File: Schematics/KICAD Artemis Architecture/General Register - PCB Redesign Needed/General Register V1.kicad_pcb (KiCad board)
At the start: 4 copper layers, 54.8 x 34.2 mm, 24 parts, among them J1 Power, J2 Bus, J3 Control, J4 A Value, U4 74LS173, U5 74LS173, U6 74LS245

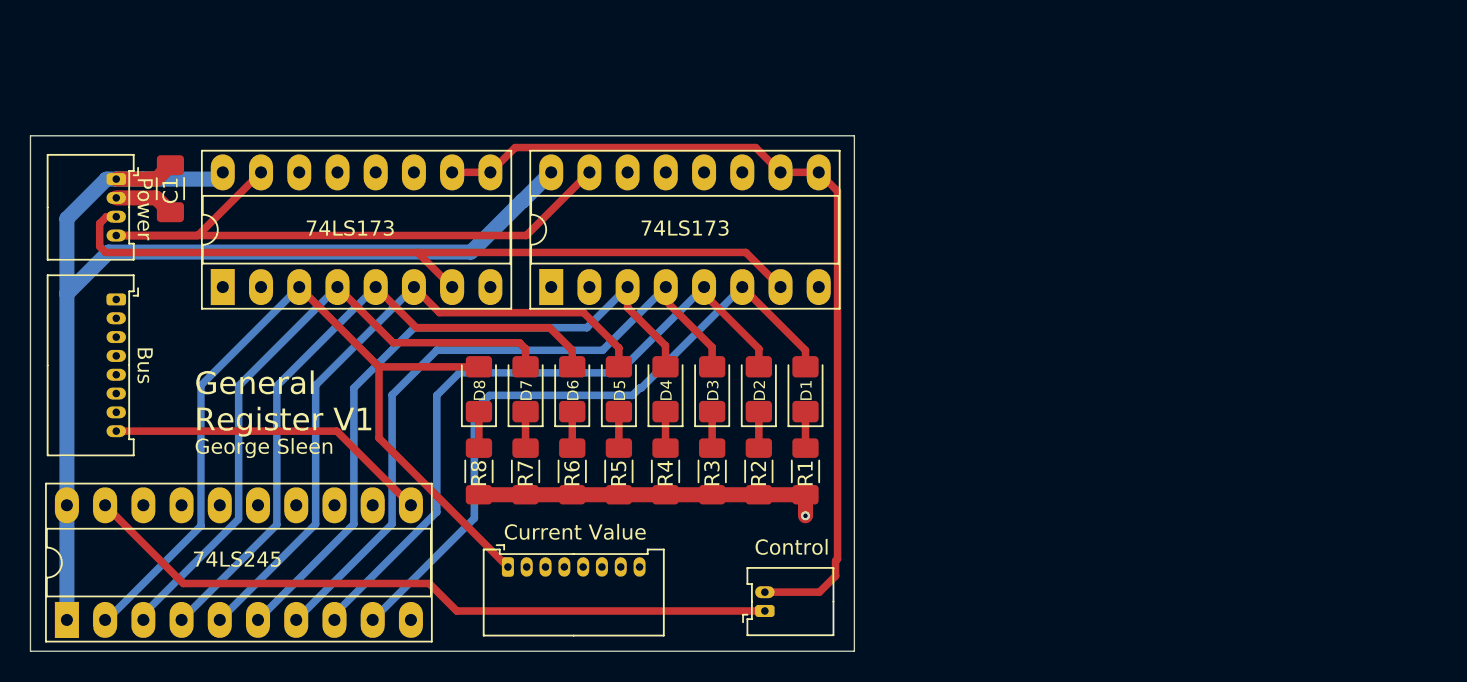
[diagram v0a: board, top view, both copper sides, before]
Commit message: Remade General Register PCB
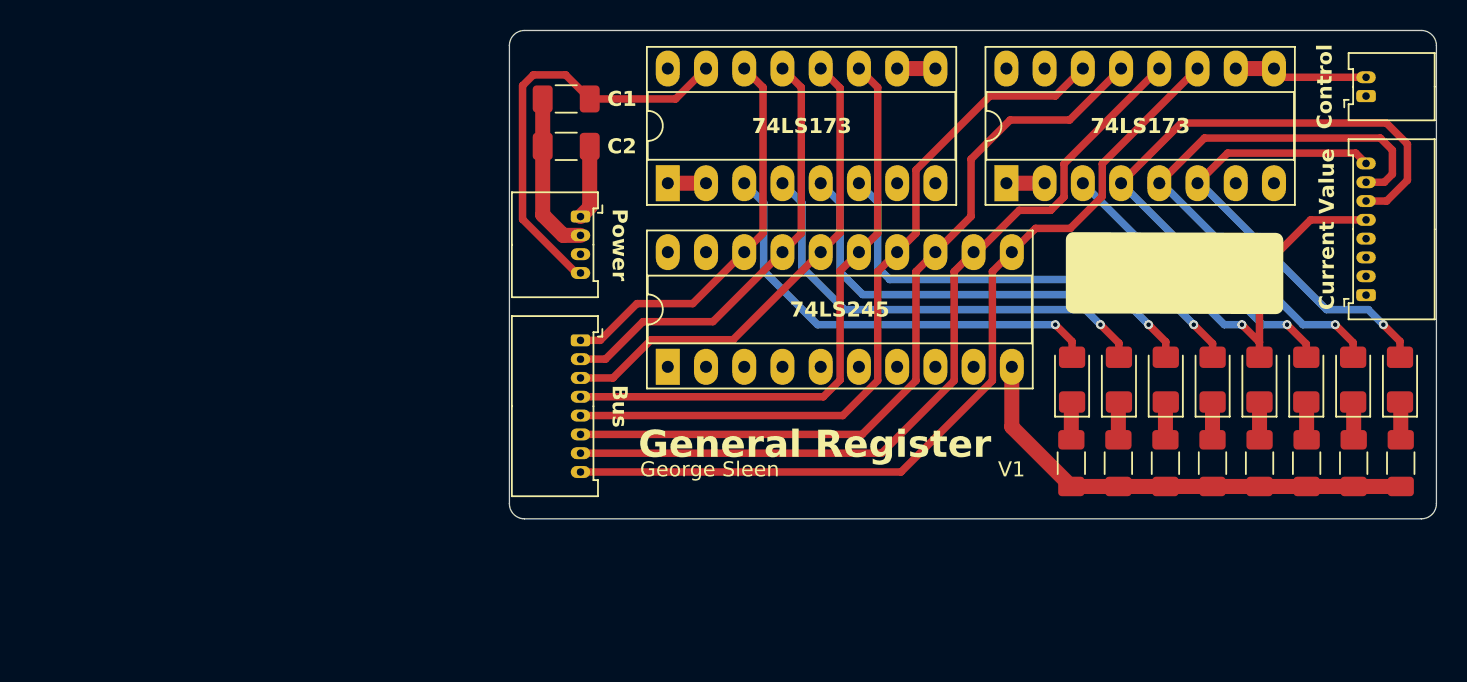
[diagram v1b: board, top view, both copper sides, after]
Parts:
- removed C3: 0.1uF, Capacitor_SMD:C_1206_3216Metric_Pad1.33x1.80mm_HandSolder
- added C1: 0.1uF, Capacitor_SMD:C_1206_3216Metric_Pad1.33x1.80mm_HandSolder, F.Cu at (126.1, 57.8)
- added C2: 0.1uF, Capacitor_SMD:C_1206_3216Metric_Pad1.33x1.80mm_HandSolder, F.Cu at (126.1, 61.0)
- J4: value A Value -> Current Value
- moved J4 59.8 mm to (179.2, 70.8), turned to 90 degrees
- moved J3 52.6 mm to (179.2, 57.6)
- moved U6 43.3 mm to (132.8, 75.6)
- moved R8 39.6 mm to (181.6, 82.0)
- moved R7 39.5 mm to (178.4, 82.0)
- moved D8 39.5 mm to (181.5, 76.5)
- moved R6 39.5 mm to (175.3, 82.0)
- moved D7 39.5 mm to (178.4, 76.5)
- moved D6 39.5 mm to (175.3, 76.5)
- moved R5 39.5 mm to (172.2, 82.0)
- moved D5 39.5 mm to (172.2, 76.5)
- moved D4 39.5 mm to (169.1, 76.5)
- moved R4 39.4 mm to (169.0, 82.0)
- moved D3 39.4 mm to (165.9, 76.5)
- moved D2 39.4 mm to (162.8, 76.5)
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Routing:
- net GNDREF: track 27.1 -> 87.2 mm, vias 1 -> 0
- net VCC: track 77.8 -> 29.4 mm
- net /A6: track 66.7 -> 108.2 mm, vias 0 -> 1
- net /A7: track 83.0 -> 113.9 mm, vias 0 -> 1
- net /A5: track 66.6 -> 97.2 mm, vias 0 -> 1
- net /A4: track 66.8 -> 94.9 mm, vias 0 -> 1
- net /~{Ain}: track 58.3 -> 32.9 mm
- net /BUS 7: track 36.8 -> 26.5 mm
- net /BUS 6: track 39.8 -> 29.6 mm
- net /BUS 5: track 42.6 -> 32.7 mm
- net /BUS 1: track 64.0 -> 54.6 mm
- net /A2: track 65.8 -> 74.1 mm, vias 0 -> 1
- net /BUS 3: track 57.6 -> 49.6 mm
- net /CLR: track 44.5 -> 52.1 mm
- net /A0: track 66.4 -> 60.5 mm, vias 0 -> 1
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- added copper zone on In1.Cu, net GNDREF
- added copper zone on In2.Cu, net VCC
- removed copper zone on In2.Cu, net GNDREF
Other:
- board size 54.8 x 34.2 mm -> 61.6 x 32.5 mm
- board text added: "General Register"
- board text added: "V1"
- board text removed: "A Value"
- board text removed: "C1"
- board text removed: "D1"
- board text removed: "D2"
- board text removed: "D3"
- board text removed: "D4"
- board text removed: "D5"
- board text removed: "D6"
- board text removed: "D7"
- board text removed: "D8"
- board text removed: "General Register V1"
- board text removed: "R1"
- board text removed: "R2"
- board text removed: "R3"
- board text removed: "R4"
- board text removed: "R5"
- board text removed: "R6"
- board text removed: "R7"
- board text removed: "R8"
